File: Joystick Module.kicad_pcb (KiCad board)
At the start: 2 copper layers, 29.5 x 23.4 mm, 2 parts, among them J1 Conn_01x05_Pin

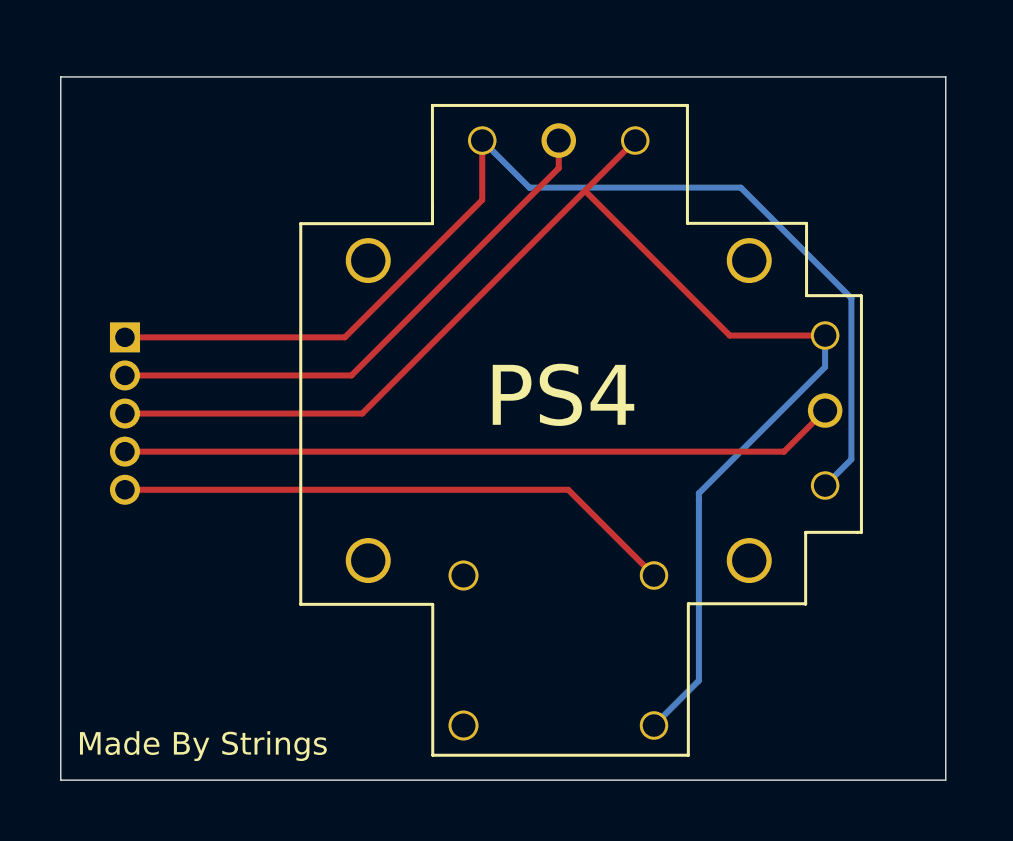
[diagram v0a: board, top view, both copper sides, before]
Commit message: Add files via upload
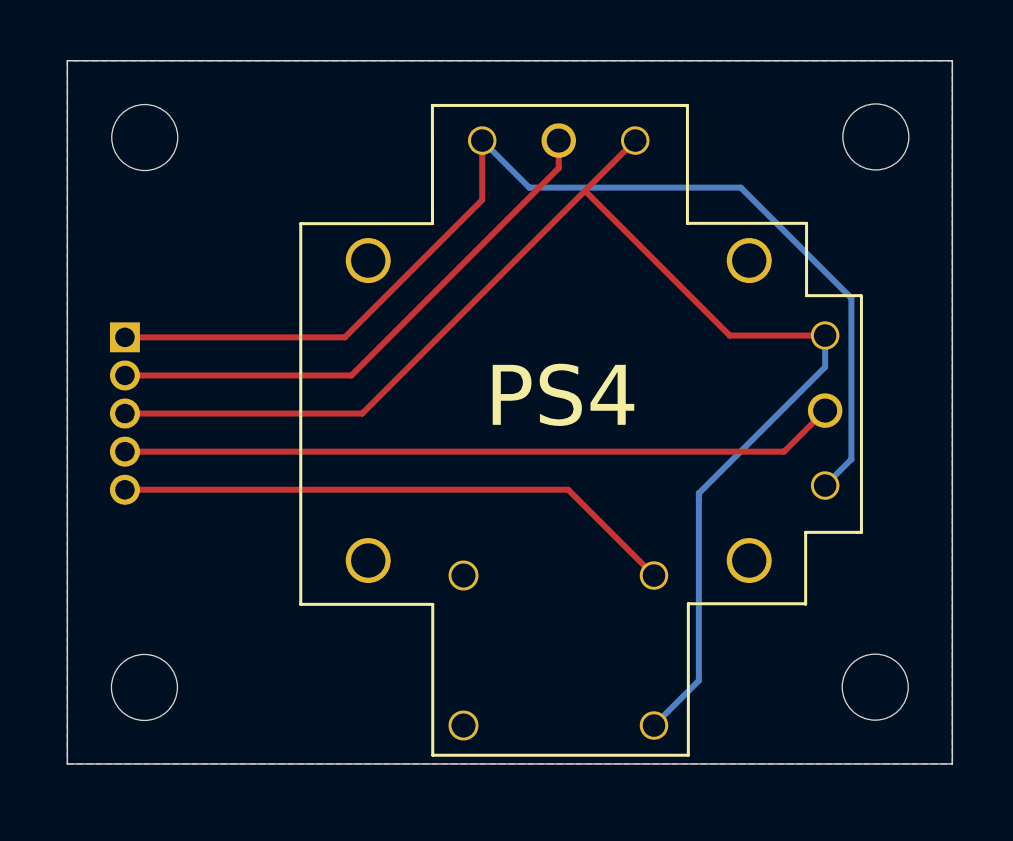
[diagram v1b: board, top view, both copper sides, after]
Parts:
- added H1: MountingHole, MountingHole:MountingHole_2.2mm_M2, F.Cu at (150.2, 109.2)
- added H2: MountingHole, MountingHole:MountingHole_2.2mm_M2, F.Cu at (125.8, 127.6)
- added H3: MountingHole, MountingHole:MountingHole_2.2mm_M2, F.Cu at (125.8, 109.3)
- added H4: MountingHole, MountingHole:MountingHole_2.2mm_M2, F.Cu at (150.2, 127.6)
- U1: renamed from PS4 Joystick
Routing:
- added copper zone on B.Cu, net GND
- added copper zone on F.Cu, net GND
